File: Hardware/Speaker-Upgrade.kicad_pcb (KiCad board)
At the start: 2 copper layers, 88.9 x 48.3 mm, 35 parts, among them J1 POWER, J2 CONN_PCB1, J3 CONN_PCB2, J4 AUDIO_JACK, U1 LM7805, U2 WIN-668, U3 AN7522N

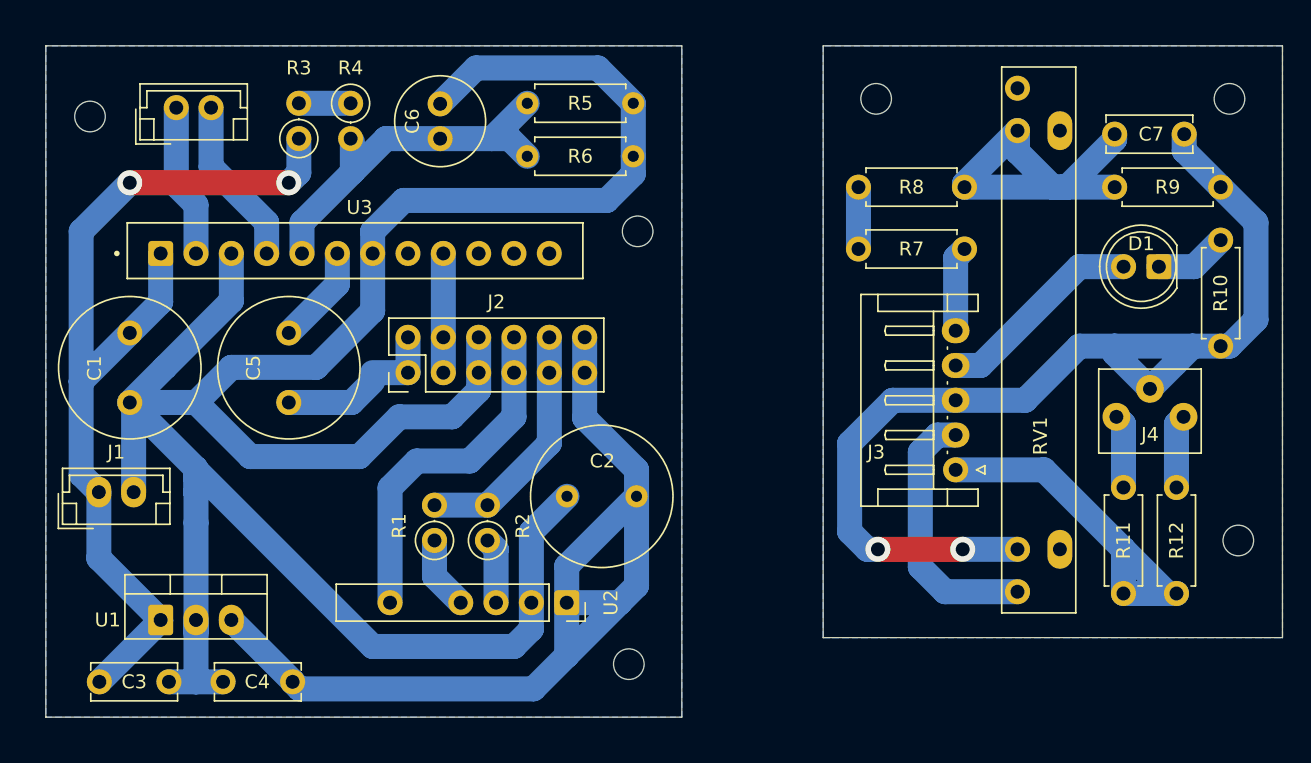
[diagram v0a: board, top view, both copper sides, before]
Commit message: Minor improvements on schematics and PCB
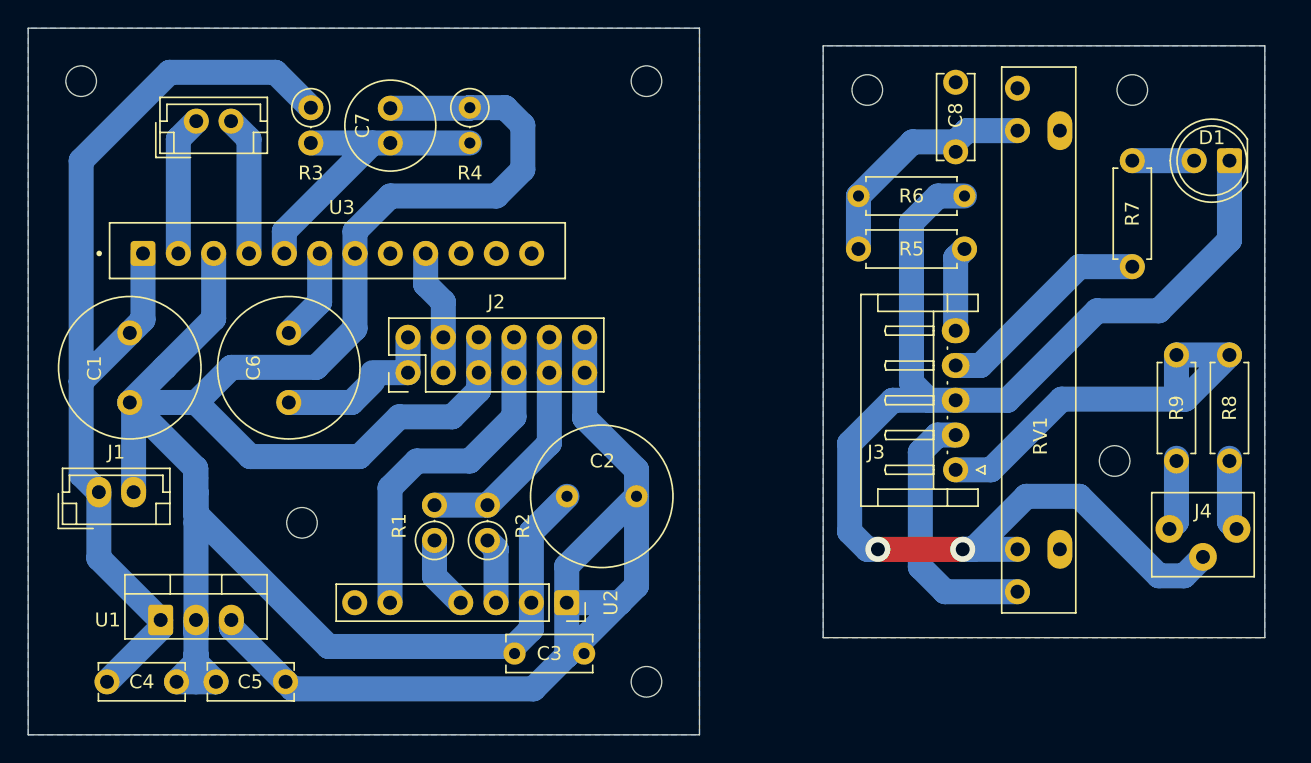
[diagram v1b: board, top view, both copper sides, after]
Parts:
- removed the R4 at (126.0, 68.9)
- removed the R8 at (162.6, 74.9)
- removed the R9 at (181.0, 74.9)
- added C3: 100nF, Capacitor_THT:C_Disc_D6.0mm_W2.5mm_P5.00mm, F.Cu at (142.8, 108.5)
- added H4: MountingHole, MountingHole:MountingHole_2.2mm_M2, F.Cu at (122.6, 99.1)
- R3: value 47K -> 68K
- R4: renamed from R5; value 1M -> 270K; footprint Resistor_THT:R_Axial_DIN0207_L6.3mm_D2.5mm_P7.62mm_Horizontal -> Resistor_THT:R_Axial_DIN0207_L6.3mm_D2.5mm_P2.54mm_Vertical
- R5: renamed from R7; value 22K -> 10K
- R6: value 330K -> 3.3K
- moved H3 41.9 mm to (147.3, 67.3)
- moved H2 32.4 mm to (147.3, 110.5)
- moved R8 18.8 mm to (189.2, 87.0), turned to -90 degrees
- moved R9 17.1 mm to (185.4, 87.0), turned to -90 degrees
- moved R6 16.4 mm to (162.6, 75.6), turned to 0 degrees
- moved R7 14.8 mm to (182.2, 73.0), turned to -90 degrees
- moved R4 11.8 mm to (134.6, 69.2), turned to -90 degrees
- moved C8 11.5 mm to (169.5, 72.4), turned to 90 degrees
- moved H7 10.6 mm to (181.0, 94.6)
- moved D1 9.16 mm to (189.2, 73.0)
- moved J4 8.92 mm to (187.3, 99.5), turned to 180 degrees
- moved H6 7.01 mm to (182.2, 67.9)
- moved C7 3.60 mm to (128.9, 71.8)
- moved H1 2.62 mm to (106.7, 67.3)
- moved R3 2.39 mm to (123.2, 69.2), turned to -90 degrees
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- renumbered C3 to C4, C4 to C5, C5 to C6, C6 to C7, C7 to C8, H4 to H5, H5 to H6, H6 to H7, R10 to R7, R11 to R8, R12 to R9
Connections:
- C8 pad 1: Net-(C7-Pad1) -> Net-(C8-Pad1)
- D1 pad 1: Net-(D1-K) -> UI_GND
- D1 pad 2: UI_LED -> Net-(D1-A)
- R3 pad 2: Net-(R3-Pad2) -> STAND_BY
- R5 pad 2: Net-(R7-Pad2) -> Net-(C8-Pad1)
- R6 pad 1: GND -> Net-(C8-Pad1)
- R6 pad 2: STAND_BY -> UI_GND
- R7 pad 1: UI_GND -> Net-(D1-A)
- R7 pad 2: Net-(D1-K) -> UI_LED
- RV1 pad 3: Net-(C7-Pad1) -> Net-(C8-Pad1)
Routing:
- net Net-(C7-Pad1): track 27.8 -> 0.00 mm
- net UI_GND: track 75.6 -> 97.6 mm
- net Net-(C8-Pad1): track 0.00 -> 17.2 mm
- net GND: track 182.9 -> 172.8 mm
- net Net-(D1-K): track 5.23 -> 0.00 mm
- net STAND_BY: track 27.2 -> 22.0 mm
- net +12V: track 68.0 -> 72.7 mm, vias 2 -> 0
- net Net-(R7-Pad2): track 4.44 -> 0.00 mm
- net Net-(D1-A): track 0.00 -> 4.44 mm
- net Net-(R3-Pad2): track 3.72 -> 0.00 mm
- net UI_AUDIO: track 26.5 -> 30.1 mm
- net CH1_OUT(-): track 12.1 -> 10.0 mm
- net CH1_OUT(+): track 11.1 -> 10.0 mm
- net UI_LED: track 15.0 -> 15.6 mm
- net VOLUME: track 8.57 -> 9.10 mm
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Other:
- board size 88.9 x 48.3 mm -> 88.9 x 50.8 mm
